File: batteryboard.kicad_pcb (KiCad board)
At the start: 2 copper layers, 46.8 x 46.8 mm, 0 parts

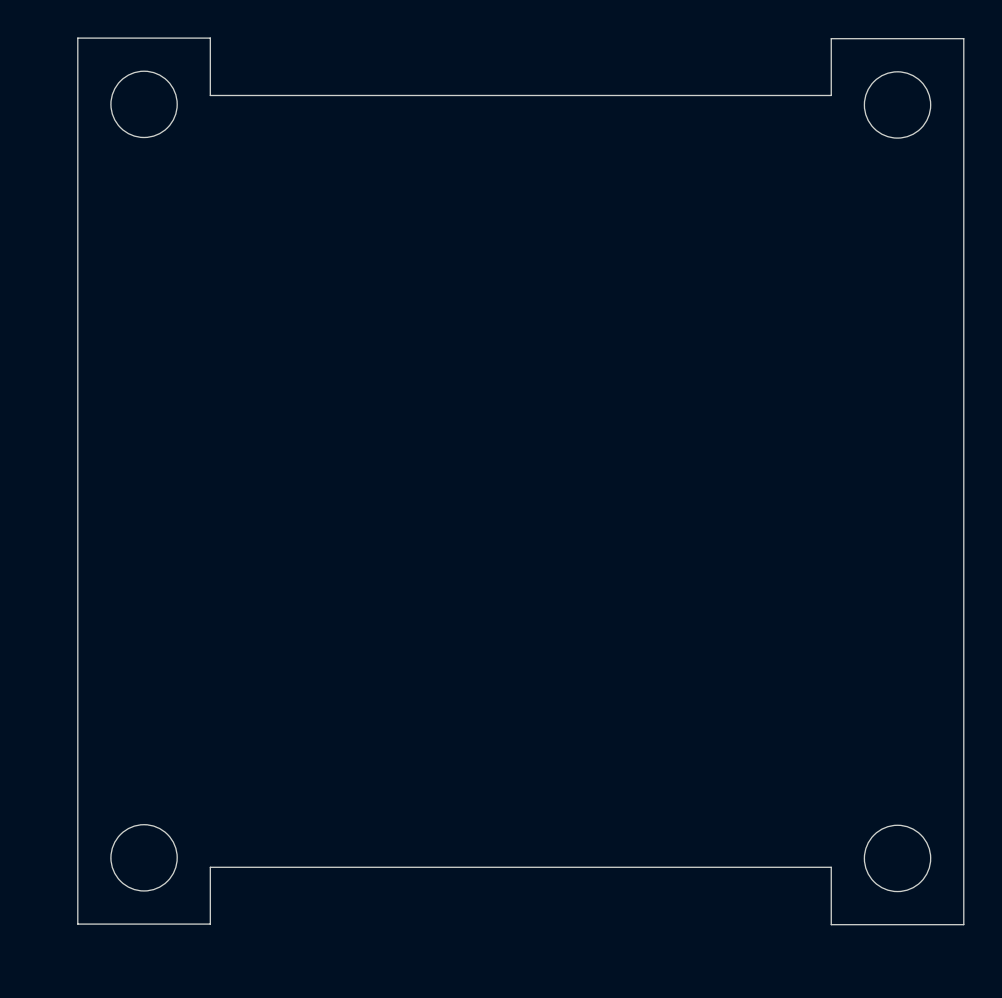
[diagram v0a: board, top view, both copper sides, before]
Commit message: completed routing
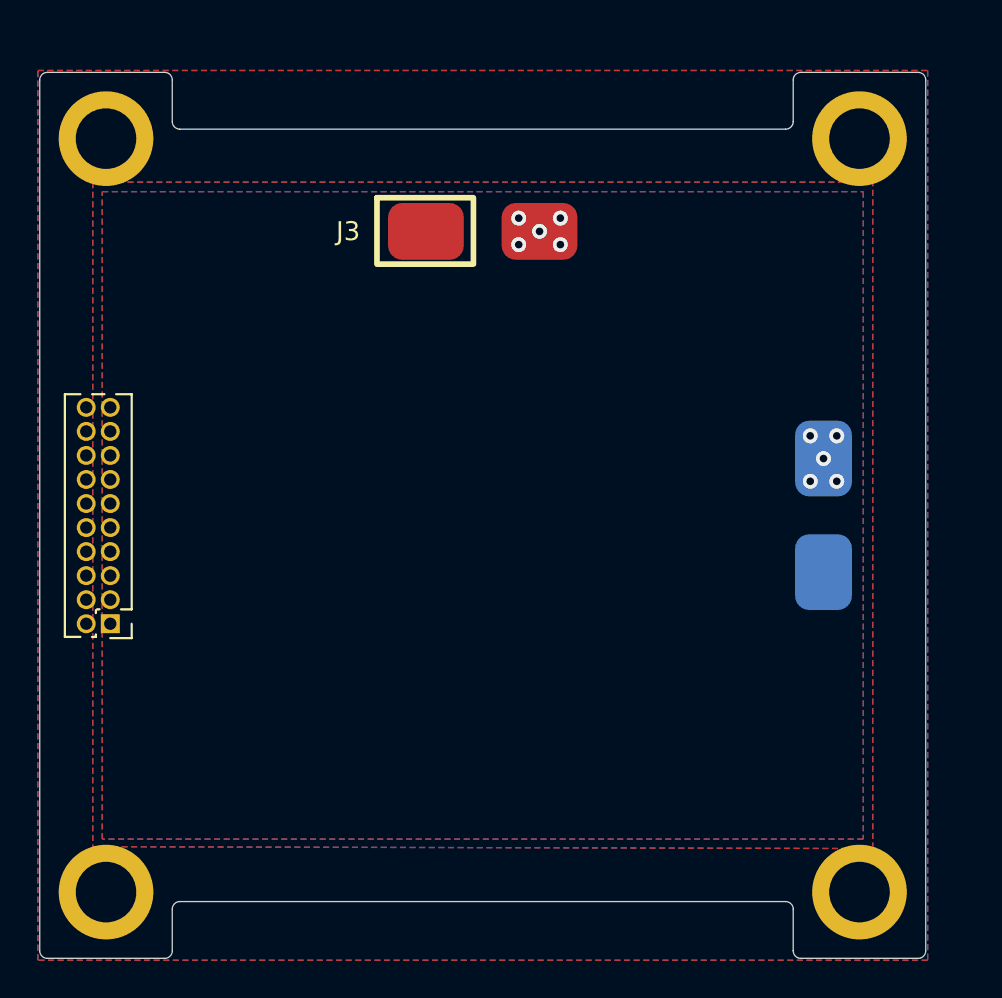
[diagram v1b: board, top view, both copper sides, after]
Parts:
- added H1: MountingHole_Pad, mainboard:MountingHole, F.Cu at (125.4, 77.9)
- added H2: MountingHole_Pad, mainboard:MountingHole, F.Cu at (165.2, 77.9)
- added H3: MountingHole_Pad, mainboard:MountingHole, F.Cu at (165.2, 117.7)
- added H4: MountingHole_Pad, mainboard:MountingHole, F.Cu at (125.4, 117.7)
- added J1: Conn 02x10 1.27mm, Connector_PinHeader_1.27mm:PinHeader_2x10_P1.27mm_Vertical, F.Cu at (125.6, 103.5)
- added J2: Conn_01x02, batteryboard:Battery Pads, B.Cu at (163.3, 97.8)
- added J3: Conn_01x02, batteryboard:Battery Pads, F.Cu at (145.3, 82.8)
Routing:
- net BATT_P_SW: vias 0 -> 5
- net BATT_N_SW: vias 0 -> 5
- added copper zone on B.Cu, net BATT_N_SW
- added copper zone on F.Cu, net BATT_P_SW
- added copper zone on B.Cu, net GND
- added copper zone on F.Cu, net GND
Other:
- outline, holes or cut-outs redrawn
